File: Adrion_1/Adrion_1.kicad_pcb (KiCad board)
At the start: 4 copper layers, 215.2 x 179.8 mm, 118 parts, among them IC1 REF1933AIDDCR, IC2 UCC21521DW, IC3 UCC21521DW, IC4 TLF80511TFV50ATMA1, J1 1705469, J2 1705469, J3 1729128, J6 M20-7821546, J7 M20-7821546, Q1 IPP111N15N3GXKSA1, Q2 IPP111N15N3GXKSA1, Q3 IPP111N15N3GXKSA1, Q5 IPP111N15N3GXKSA1, U3 NUCLEO-G431KB, U4 TPS7A2033PDBVR, U5 CKSR_6-NP

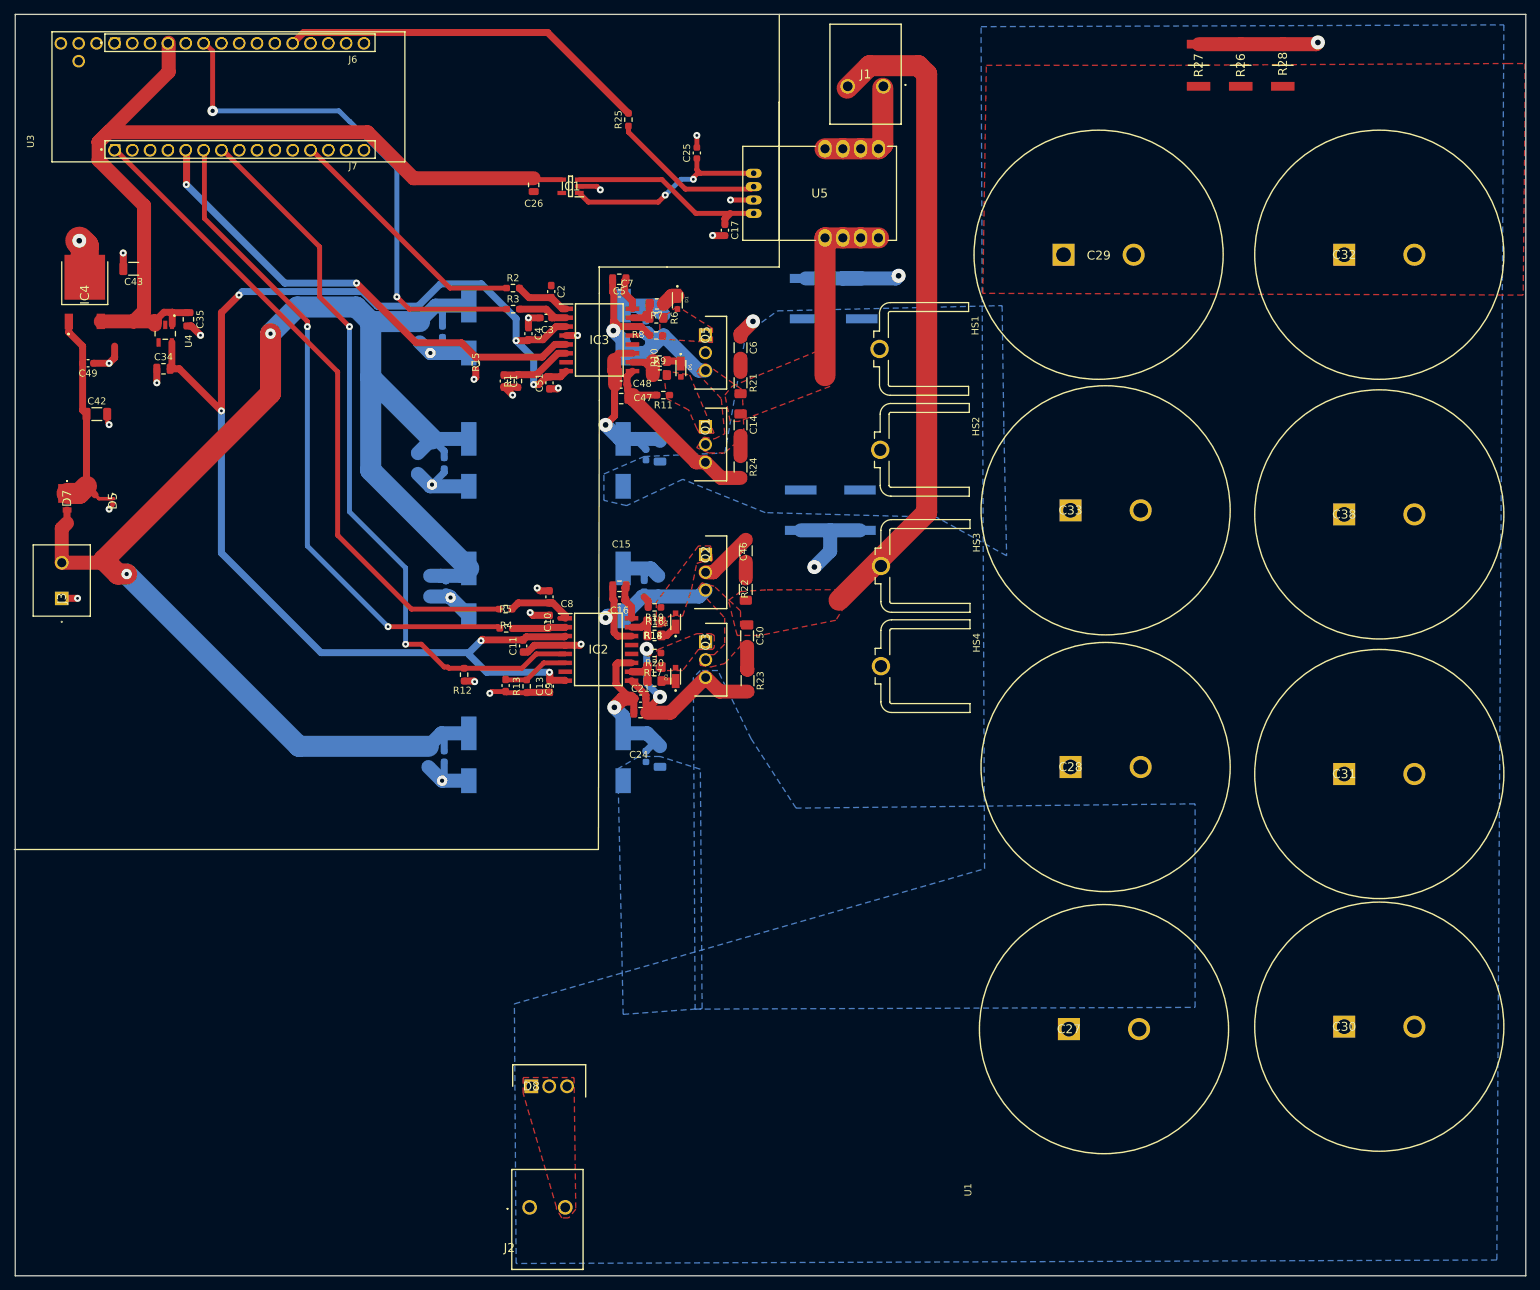
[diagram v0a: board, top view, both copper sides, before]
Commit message: FirstPrototype
First Prototype sent
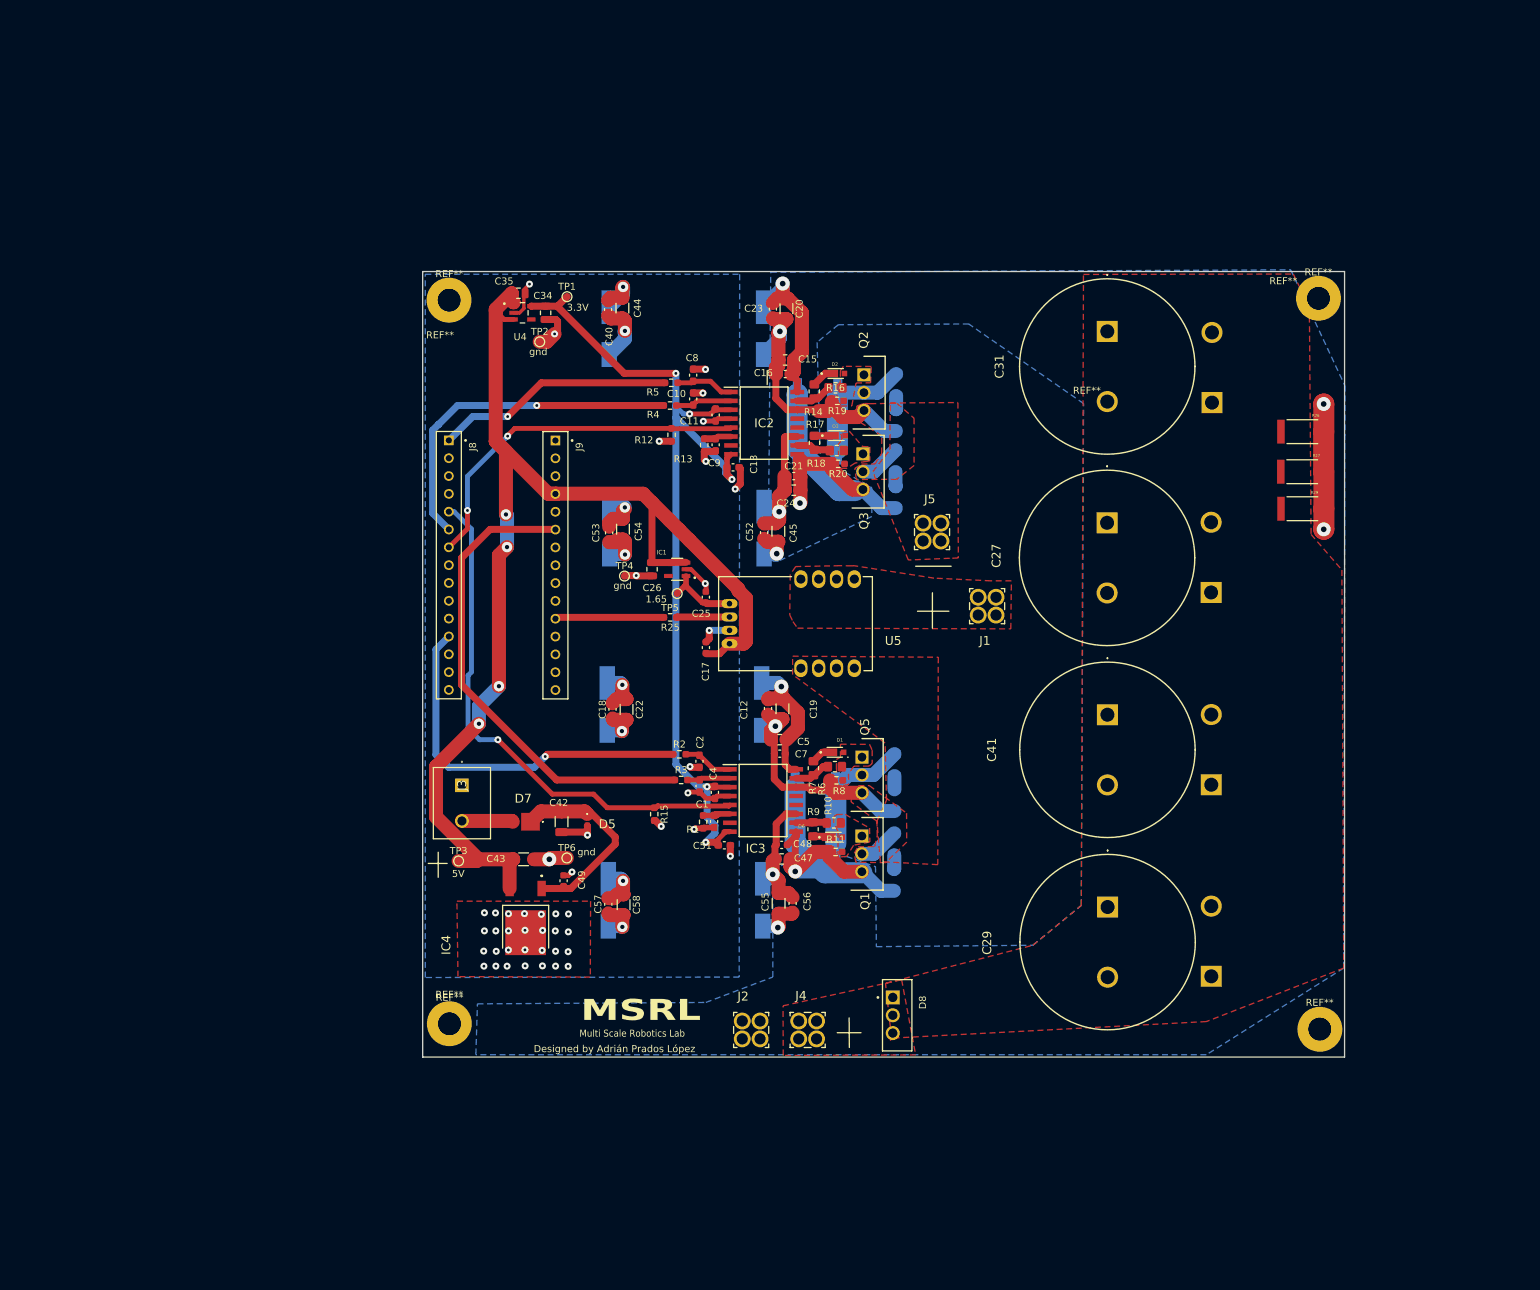
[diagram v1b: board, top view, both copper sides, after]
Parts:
- removed C33: B43547F2108M067, CAPPRD1000W190D3550H4200:CAPPRD1000W190D3550H4200
- removed C38: 1000u, CAPPRD1000W190D3550H4200:CAPPRD1000W190D3550H4200
- removed HS1, HS2, HS3, HS4: 577202B04000G, HSINK_577202B04000G:HSINK_577202B04000G
- removed J6, J7: M20-7821546, HARWIN_M20-7821546:HARWIN_M20-7821546
- removed R28: CRCW251215K0FKEG, RESC6332X70N:RESC6332X70N
- removed U1: ~, 1705469:Untitled
- removed U3: NUCLEO-G431KB, MODULE_NUCLEO-G431KB:MODULE_NUCLEO-G431KB
- added C41: LGU2D102MELA, LGU2D102MELA:LGU2D102MELA, F.Cu at (180.0, 111.0)
- added C60: LGU2D102MELA, LGU2D102MELA:LGU2D102MELA, B.Cu at (194.8, 148.3)
- added J4: 7462810, 7462810:7462810, F.Cu at (137.3, 156.0)
- added J5: 7462810, 7462810:7462810, F.Cu at (155.0, 85.0)
- added J8: 6-534237-3, TE_6-534237-3:TE_6-534237-3, F.Cu at (86.2, 89.7)
- added J9: 6-534237-3, TE_6-534237-3:TE_6-534237-3, F.Cu at (101.3, 89.7)
- added R29: CRGP2512F15K, RESC6332X65N:RESC6332X65N, F.Cu at (207.8, 81.7)
- added REF**: MountingHole_3.2mm_M3_DIN965_Pad, MountingHole:MountingHole_3.2mm_M3_DIN965_Pad, F.Cu at (86.3, 155.1)
- added REF**: MountingHole_3.2mm_M3_DIN965_Pad, MountingHole:MountingHole_3.2mm_M3_DIN965_Pad, F.Cu at (210.1, 51.7)
- added REF**: MountingHole_3.2mm_M3_DIN965_Pad, MountingHole:MountingHole_3.2mm_M3_DIN965_Pad, F.Cu at (210.2, 155.8)
- added REF**: MountingHole_3.2mm_M3_DIN965_Pad, MountingHole:MountingHole_3.2mm_M3_DIN965_Pad, F.Cu at (86.2, 52.0)
- added REF**: MountingHole_3.2mm_M3_Pad, MountingHole:MountingHole_3.2mm_M3_Pad, F.Cu at (86.2, 52.0)
- added REF**: MountingHole_3.2mm_M3_Pad, MountingHole:MountingHole_3.2mm_M3_Pad, F.Cu at (210.1, 51.7)
- added REF**: MountingHole_3.2mm_M3_Pad, MountingHole:MountingHole_3.2mm_M3_Pad, F.Cu at (86.2, 155.1)
- added REF**: MountingHole_3.2mm_M3_Pad, MountingHole:MountingHole_3.2mm_M3_Pad, F.Cu at (210.3, 155.9)
- added TP1: TestPoint, TestPoint:TestPoint_Pad_D1.0mm, F.Cu at (103.0, 51.5)
- added TP2: TestPoint, TestPoint:TestPoint_Pad_D1.0mm, F.Cu at (99.1, 57.9)
- added TP3: TestPoint, TestPoint:TestPoint_Pad_D1.0mm, F.Cu at (87.5, 131.9)
- added TP4: TestPoint, TestPoint:TestPoint_Pad_D1.0mm, F.Cu at (111.2, 91.3)
- added TP5: TestPoint, TestPoint:TestPoint_Pad_D1.0mm, F.Cu at (118.7, 93.8)
- added TP6: TestPoint, TestPoint:TestPoint_Pad_D1.0mm, F.Cu at (103.0, 131.5)
- C12, C18, C19, C20, C22, C23, C40, C44, C45, C52, C53, C54, C55, C56, C57, C58: moved to F.Cu
- C14, C46, C50, C6, R21, R22, R23, R24: moved to B.Cu
- C27, C29, C31: value B43547F2108M067 -> LGU2D102MELA; footprint CAPPRD1000W190D3550H4200:CAPPRD1000W190D3550H4200 -> LGU2D102MELA:LGU2D102MELA
- C28, C30, C32: value B43547F2108M067 -> LGU2D102MELA; footprint CAPPRD1000W190D3550H4200:CAPPRD1000W190D3550H4200 -> LGU2D102MELA:LGU2D102MELA; moved to B.Cu
- D8: value STPS20200CTN -> SDT40A120CT; footprint TO255P460X1020X1905-3P:TO255P460X1020X1905-3P -> TO254P1066X482X2286-3:TO254P1066X482X2286-3
- J1, J2: value 1705469 -> 7462810; footprint 1705469:1705469 -> 7462810:7462810
- R26, R27: value CRCW251215K0FKEG -> CRGP2512F15K; footprint RESC6332X70N:RESC6332X70N -> RESC6332X65N:RESC6332X65N
- moved IC4 107.6 mm to (97.1, 139.1), turned to 90 degrees
- moved C43 100.8 mm to (96.8, 131.7), turned to 0 degrees
- moved C49 100.2 mm to (102.5, 134.7), turned to -90 degrees
- moved C29 93.2 mm to (180.0, 138.4), turned to -90 degrees
- moved C30 90.9 mm to (194.9, 66.6), turned to 90 degrees
- moved C42 88.1 mm to (102.2, 126.3), turned to -90 degrees
- moved D5 81.6 mm to (105.9, 126.2)
- moved D7 80.0 mm to (97.1, 126.3), turned to 180 degrees
- moved C39 77.9 mm to (138.4, 129.4), turned to 0 degrees
- moved C32 77.9 mm to (194.8, 121.0), turned to 90 degrees
- moved J1 75.5 mm to (162.9, 95.6), turned to 0 degrees
- moved C27 72.4 mm to (180.0, 83.7), turned to -90 degrees
- moved C31 71.5 mm to (180.0, 56.4), turned to -90 degrees
- moved R3 71.2 mm to (119.3, 120.3)
- moved R25 71.2 mm to (117.7, 97.2), turned to 180 degrees
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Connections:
- J1 pad 2: Net-(IC2-VSSA) -> Net-(U5-OUT_1)
- J2 pad 2: Net-(D8-Pad1) -> GNDPWR
- R26 pad 1: GNDPWR -> HV
- R26 pad 2: HV -> GNDPWR
- R27 pad 1: GNDPWR -> HV
- R27 pad 2: HV -> GNDPWR
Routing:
- net 12V: track 229.3 -> 34.6 mm, vias 2 -> 4
- net Net-(IC2-VSSA): track 121.8 -> 45.1 mm
- net PWM_BH: track 95.5 -> 34.2 mm, vias 0 -> 1
- net 3.3V: track 191.3 -> 131.3 mm, vias 6 -> 5
- net EN_B: track 106.3 -> 51.7 mm
- net PWM_BL: track 94.9 -> 49.5 mm, vias 2 -> 1
- net GNDPWR: track 80.4 -> 123.4 mm, vias 3 -> 6
- net I_Sense: track 53.1 -> 15.5 mm
- net Net-(IC3-VSSA): track 61.9 -> 39.2 mm
- net 1.65V: track 29.6 -> 10.6 mm, vias 2 -> 0
- net 5V: track 160.6 -> 178.4 mm, vias 0 -> 4
- net PWM_AH: track 36.0 -> 52.9 mm, vias 0 -> 1
- net Net-(U5-OUT_1): track 16.5 -> 0.00 mm
- net Net-(U5-VOUT): track 22.2 -> 7.56 mm
- net GND: track 106.0 -> 93.7 mm, vias 26 -> 51
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- added copper zone on In2.Cu, net 12V
- added copper zone on B.Cu, net GND
- added copper zone on F.Cu, net GND
- added copper zone on F.Cu, net Net-(U5-OUT_1)
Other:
- board size 215.2 x 179.8 mm -> 131.4 x 111.9 mm
- board text added: "1.65"
- board text added: "3.3V"
- board text added: "5V"
- board text added: "Designed by Adrián Prados López"
- board text added: "MSRL"
- board text added: "Multi Scale Robotics Lab"
- board text added: "PS2"
- board text added: "gnd"
